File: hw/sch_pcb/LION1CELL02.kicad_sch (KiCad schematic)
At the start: 90 parts, among them J1 USBC_USB4105-GF-A, J2 HEADER_2x03, J3 HEADER_1x04, Q1 BSS83P, Q2 BC807-25, Q3 BC807-25, SW1 SKRTLAE010, U1 BQ34Z100, U2 BQ25628E, U3 TPS631000DRLR, U4 SN74HC164P, U5 BQ29700DSER

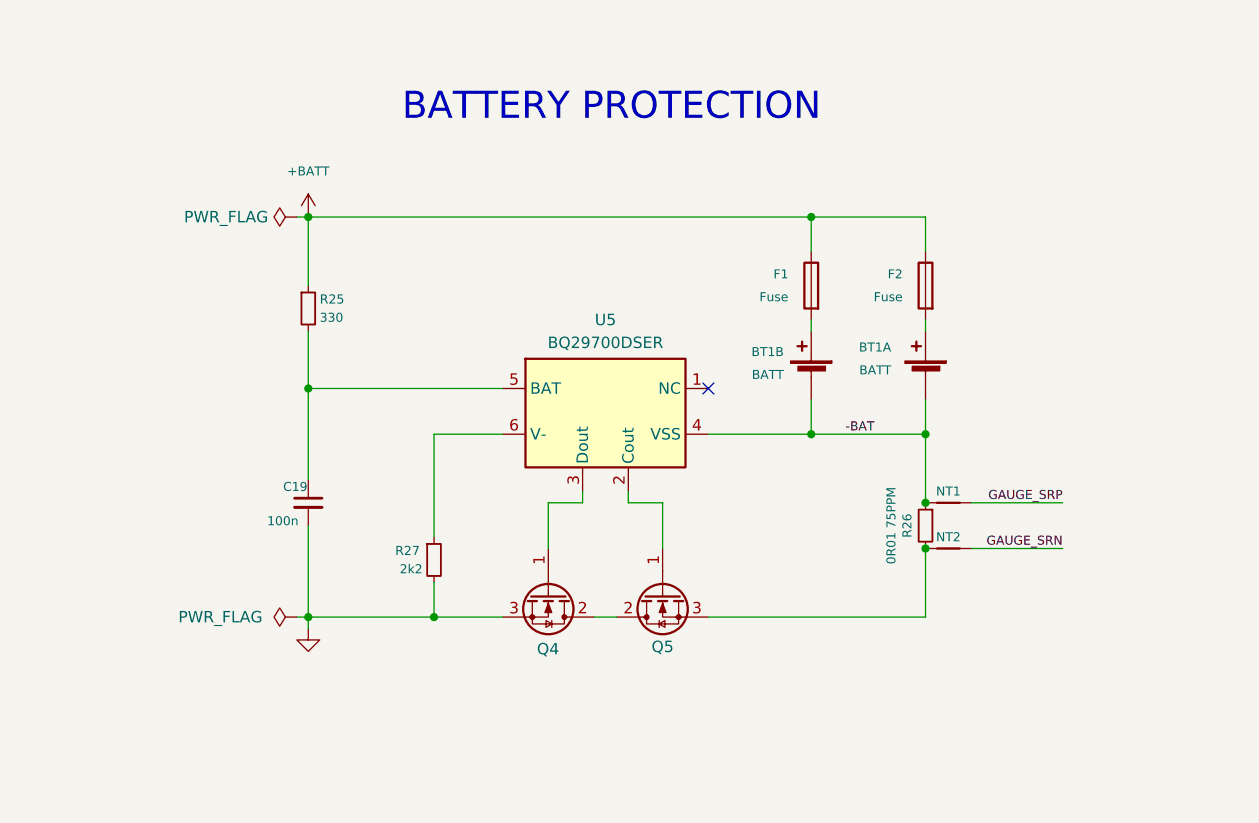
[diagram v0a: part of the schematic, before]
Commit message: Update pcb
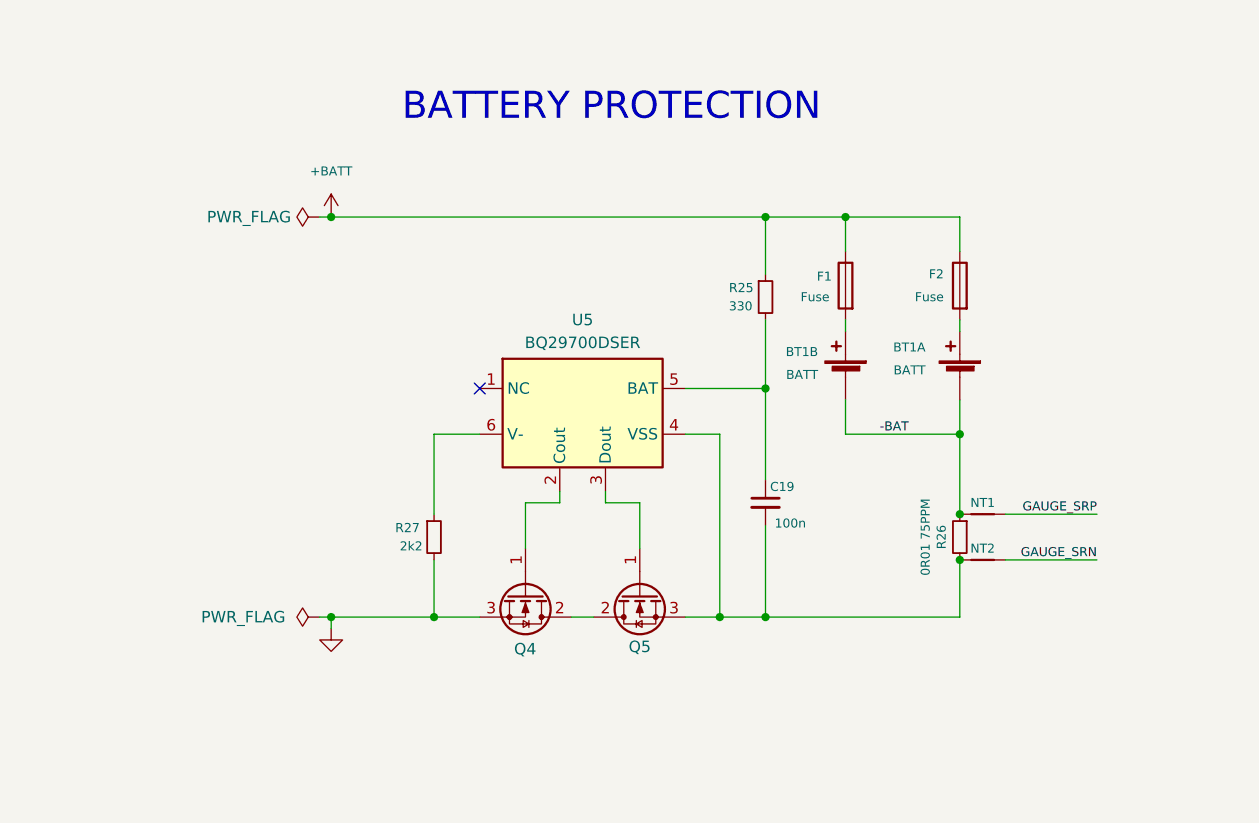
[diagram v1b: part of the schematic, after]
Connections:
- net -BAT: no longer U5.4 (VSS)
- net GND: no longer C19.2
- net at Q5.1 (G): now also U5.3 (Dout); no longer U5.2 (Cout)
- net at NT2.2, Q5.3 (S), R26.2: now also C19.2, U5.4 (VSS)
- net at Q4.1 (G): now also U5.2 (Cout); no longer U5.3 (Dout)
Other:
- moved on the sheet: BT1A, BT1B, C19, F1, F2, NT1, NT2, Q4, Q5, R25, R26, R27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
